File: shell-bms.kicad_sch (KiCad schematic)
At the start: 0 parts

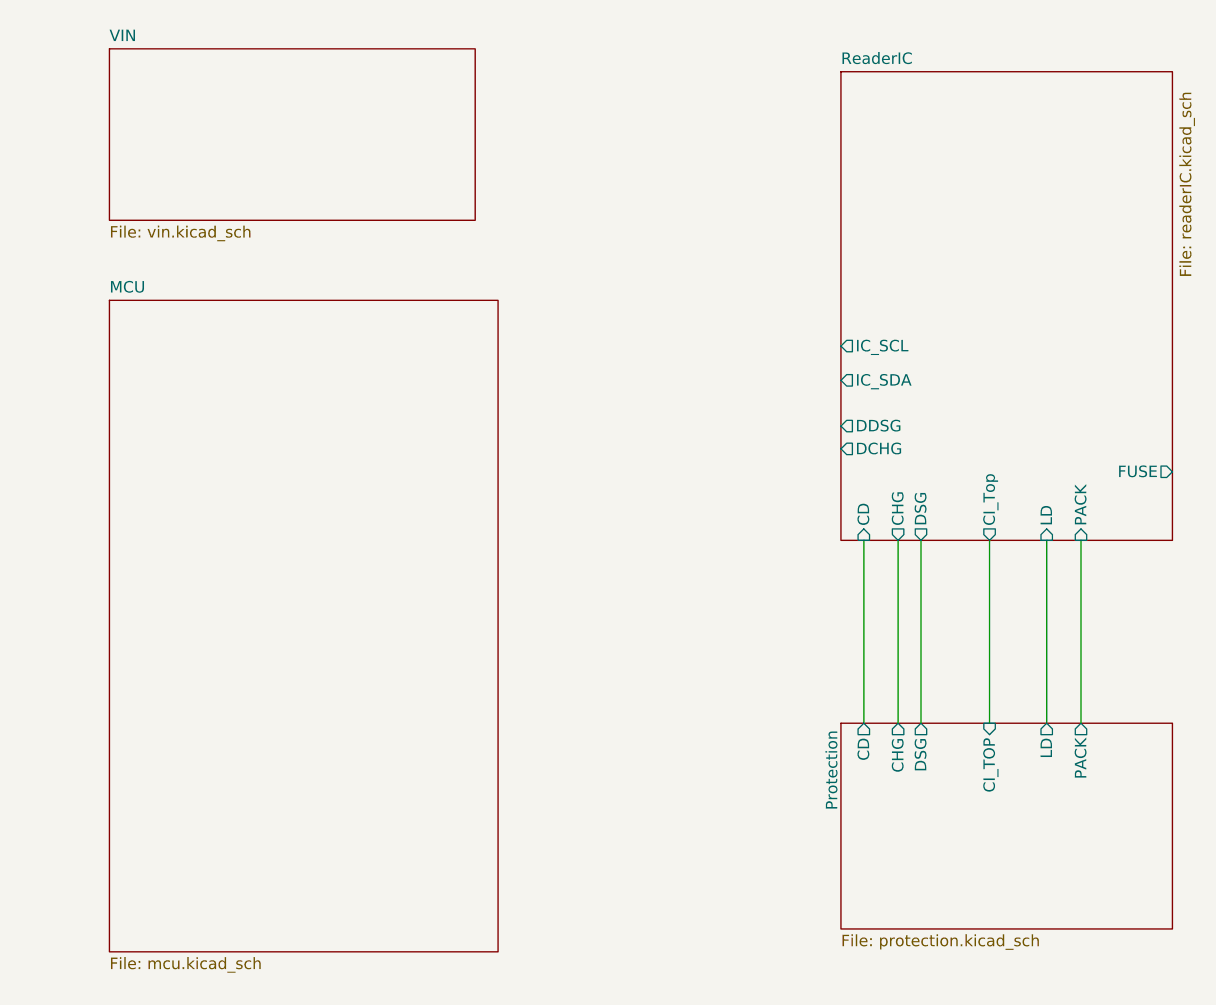
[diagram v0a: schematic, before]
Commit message: lots of lots changes. Schematic done NEEDS Review
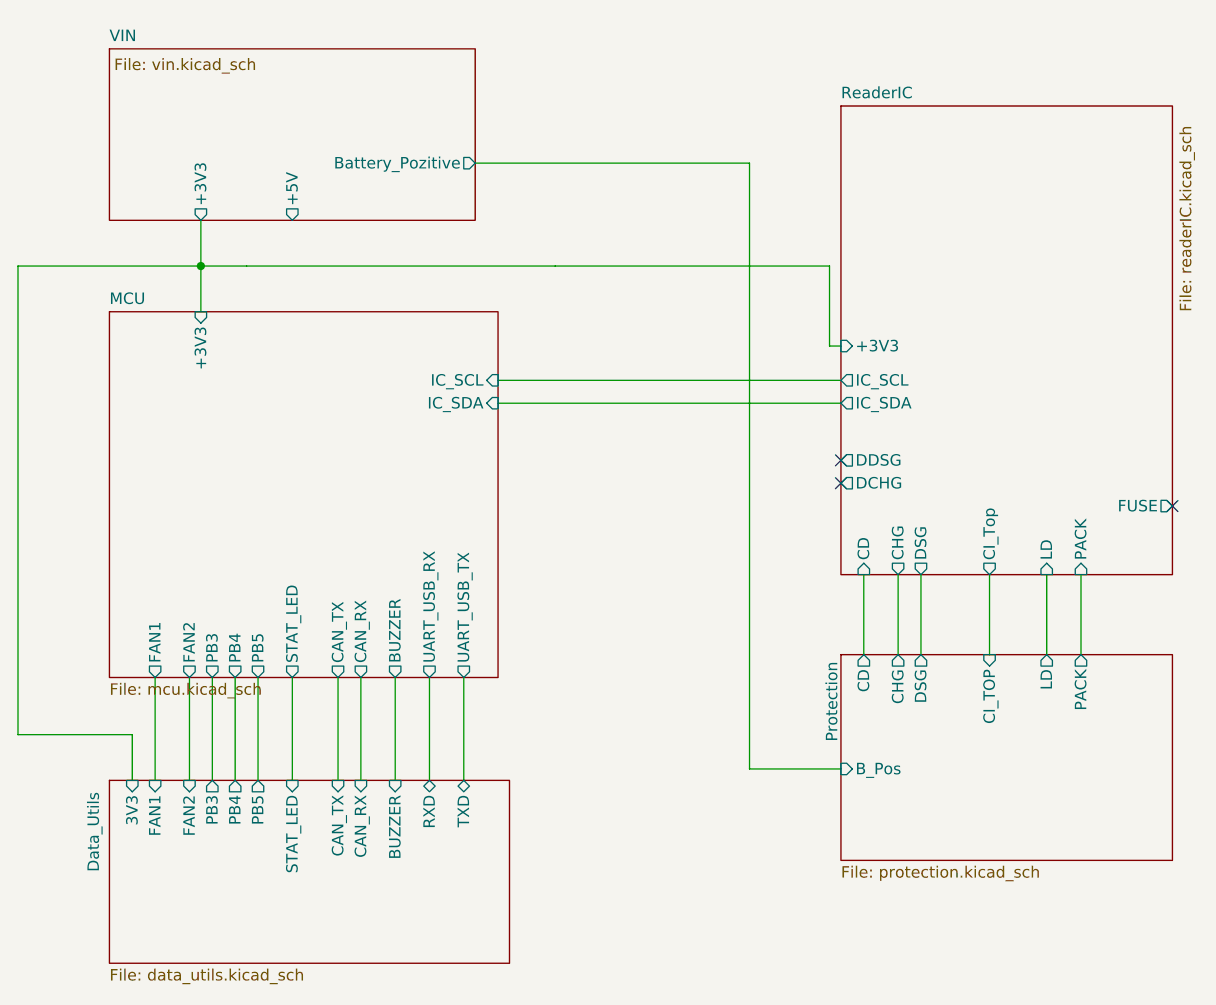
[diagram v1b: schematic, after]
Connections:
- no-connect marks 0 -> 3
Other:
- added sheet Data_Utils (data_utils.kicad_sch)
- sheet MCU ports: added +3V3, BUZZER, CAN_RX, CAN_TX, FAN1, FAN2, IC_SCL, IC_SDA, PB3, PB4, PB5, STAT_LED, UART_USB_RX, UART_USB_TX; removed none
- sheet Protection ports: added B_Pos; removed none
- sheet ReaderIC ports: added +3V3; removed none
- sheet VIN ports: added +3V3, +5V, Battery_Pozitive; removed none
- company: (none) -> Pehlivan Team
- title: (none) -> Pehli-Shell-BMS
